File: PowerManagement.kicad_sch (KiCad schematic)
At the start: 3 parts, among them J2 USB_C_Receptacle_USB2.0_16P

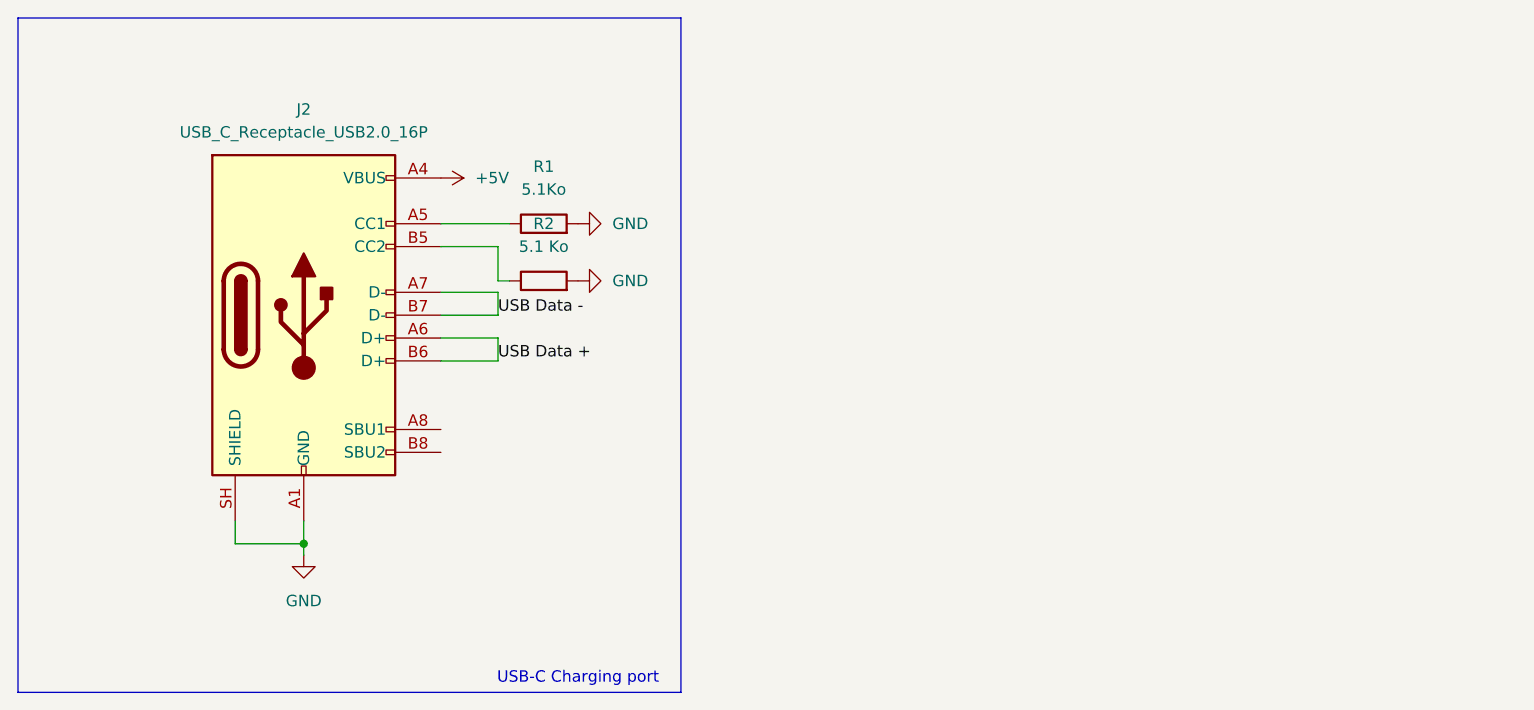
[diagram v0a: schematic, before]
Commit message: fixing project files
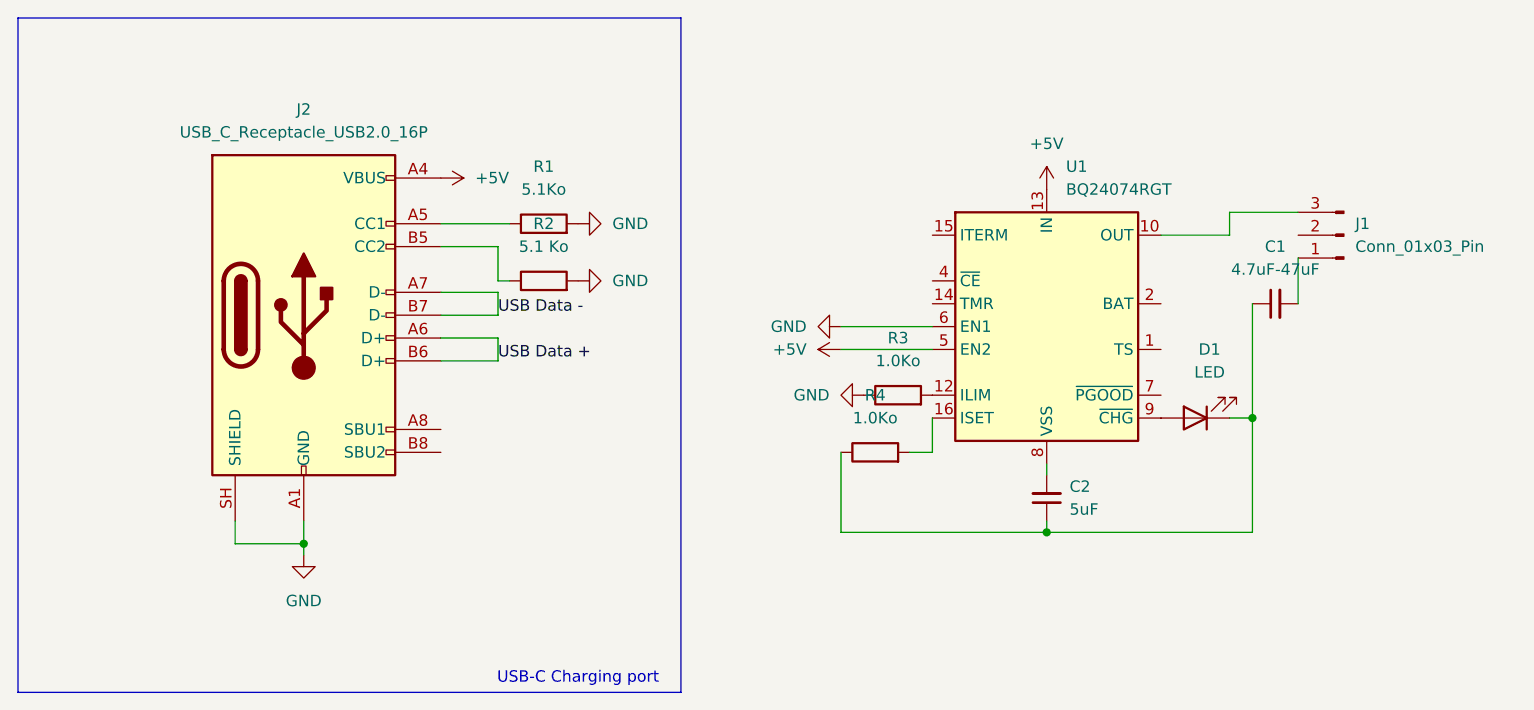
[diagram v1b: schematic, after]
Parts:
- added C1: 4.7uF-47uF, symbol Device:C_Small
- added C2: 5uF, symbol Device:C_Small
- added D1: LED, symbol Device:LED
- added J1: Conn_01x03_Pin, symbol Connector:Conn_01x03_Pin
- added R3, R4: 1.0Ko, symbol Device:R
- added U1: BQ24074RGT, Package_DFN_QFN:VQFN-16-1EP_3x3mm_P0.5mm_EP1.6x1.6mm, symbol Battery_Management:BQ24074RGT
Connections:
- net +5V: now also U1.13 (IN), U1.5 (EN2)
- net GND: now also R3.1, U1.6 (EN1)
- new net: C1.1, C2.1, D1.1 (K), R4.1
- new net: C2.2, U1.17 (VSS), U1.8 (VSS)
- new net: R3.2, U1.12 (ILIM)
- new net: J1.3 (Pin_3), U1.10 (OUT), U1.11 (OUT)
- new net: R4.2, U1.16 (ISET)
- new net: U1.2 (BAT), U1.3 (BAT)
- new net: D1.2 (A), U1.9 (~{CHG})
- new net: C1.2, J1.1 (Pin_1)
